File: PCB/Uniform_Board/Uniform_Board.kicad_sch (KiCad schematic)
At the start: 140 parts

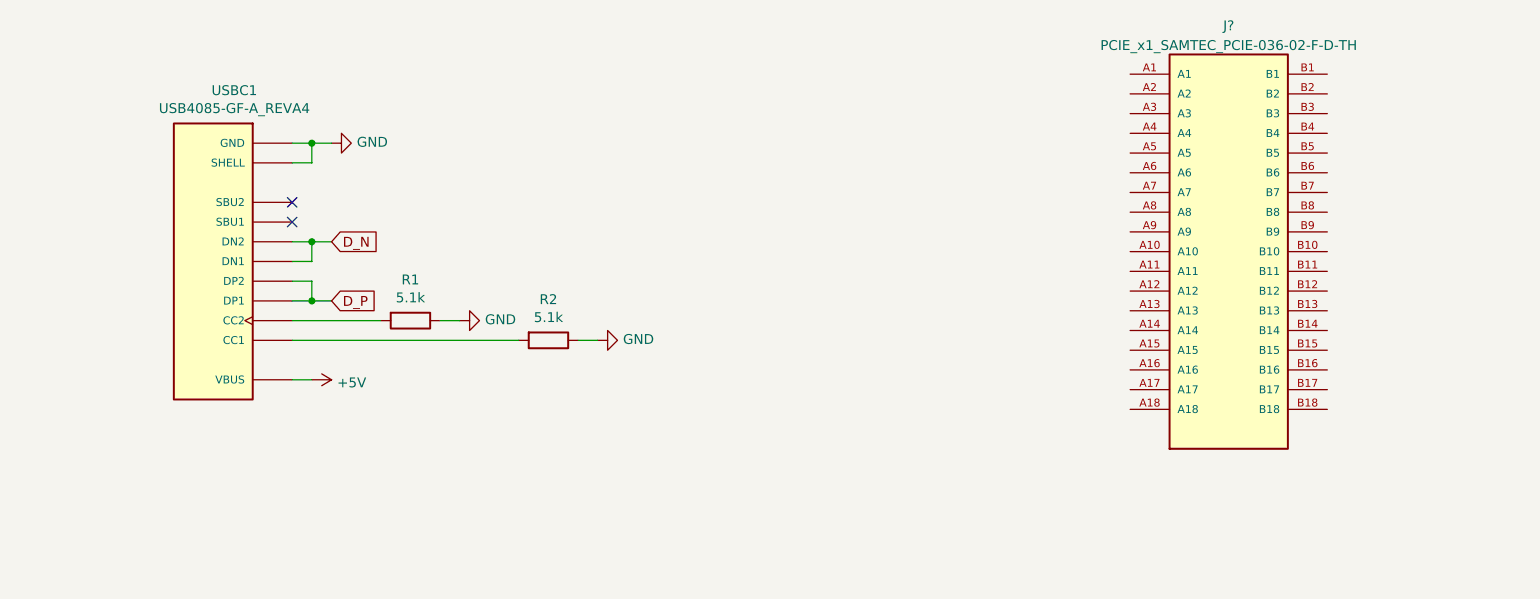
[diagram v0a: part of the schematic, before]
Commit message: completed uniform_board schematic
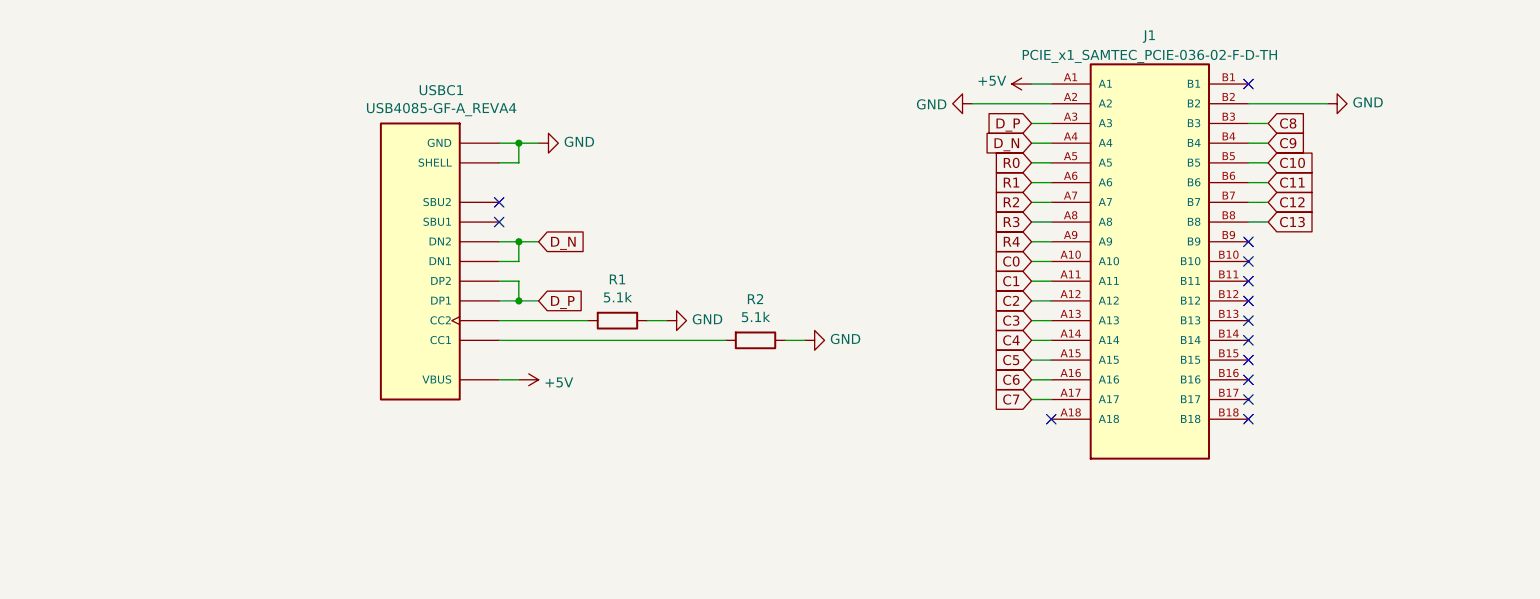
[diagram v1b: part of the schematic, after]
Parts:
- gave numbers to parts that had none: 1
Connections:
- net +5V: now also J1.A1
- net C0: now also J1.A10
- net C1: now also J1.A11
- net C10: now also J1.B5
- net C11: now also J1.B6
- net C12: now also J1.B7
- net C13: now also J1.B8
- net C2: now also J1.A12
- net C3: now also J1.A13
- net C4: now also J1.A14
- net C5: now also J1.A15
- net C6: now also J1.A16
- net C7: now also J1.A17
- net C8: now also J1.B3
- net C9: now also J1.B4
- net D_N: now also J1.A4
- net D_P: now also J1.A3
- net GND: now also J1.A2, J1.B2
- net R0: now also J1.A5
- net R1: now also J1.A6
- net R2: now also J1.A7
- net R3: now also J1.A8
- net R4: now also J1.A9
- no-connect marks 2 -> 14
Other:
- moved on the sheet: J1, R1, R2, USBC1
